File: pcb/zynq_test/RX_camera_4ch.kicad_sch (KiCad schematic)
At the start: 39 parts, among them J1601 SFW15R-2STE1LF, U1601 TCA9406DC, U1602 SN75DPHY440

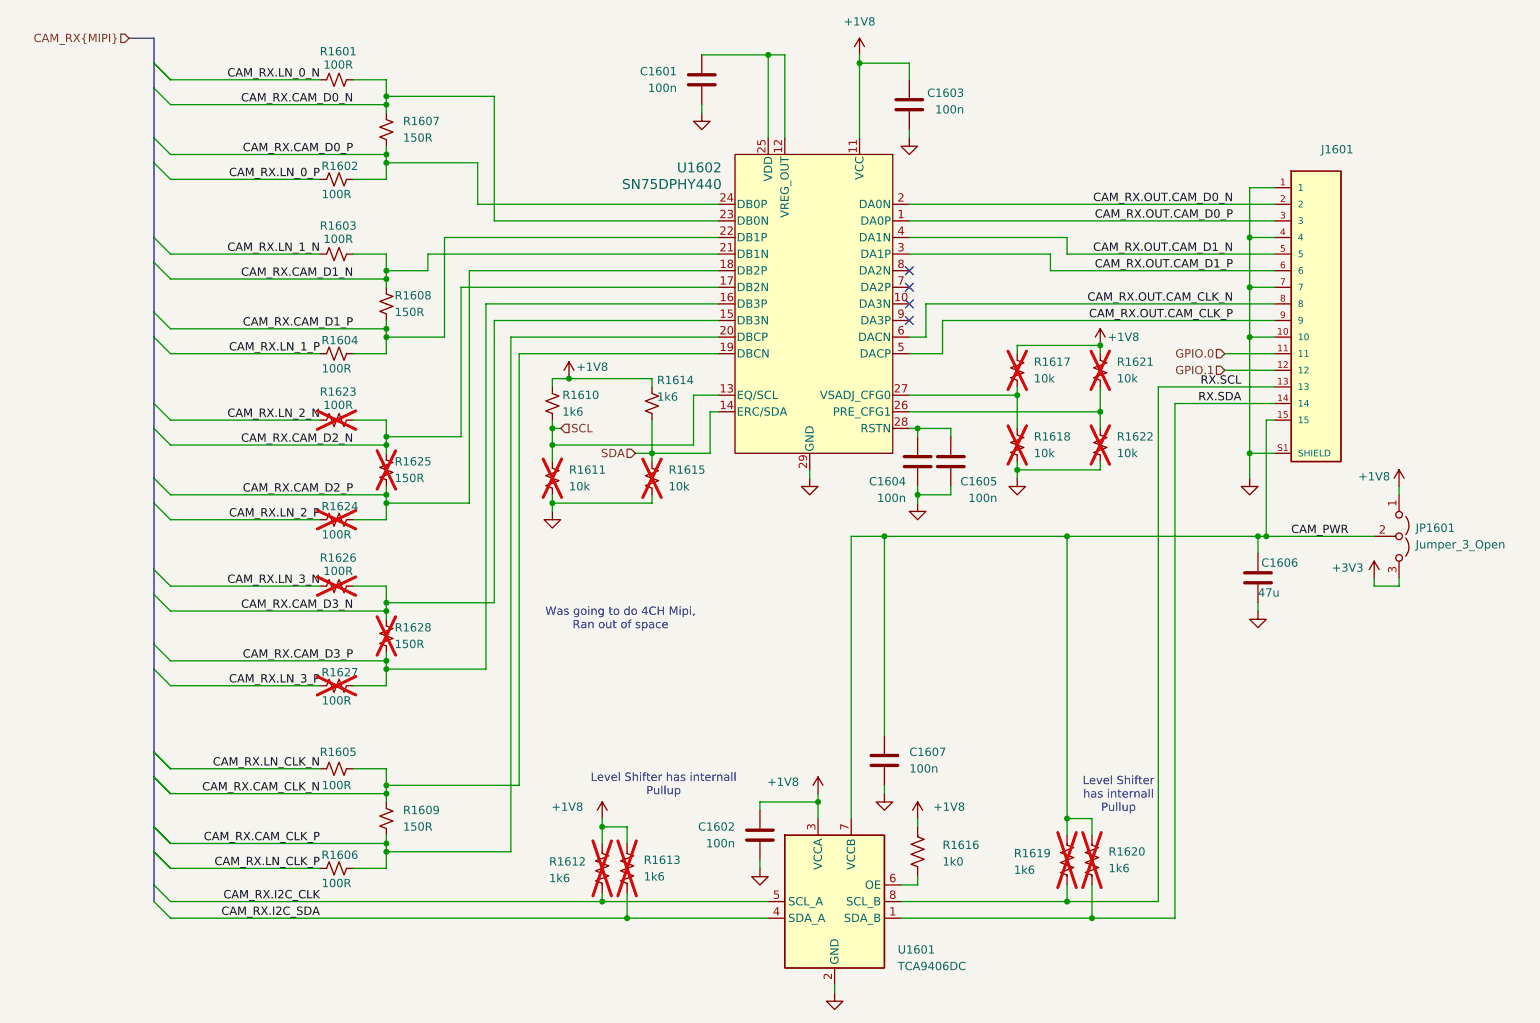
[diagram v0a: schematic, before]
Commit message: Version sent to JLCPCB
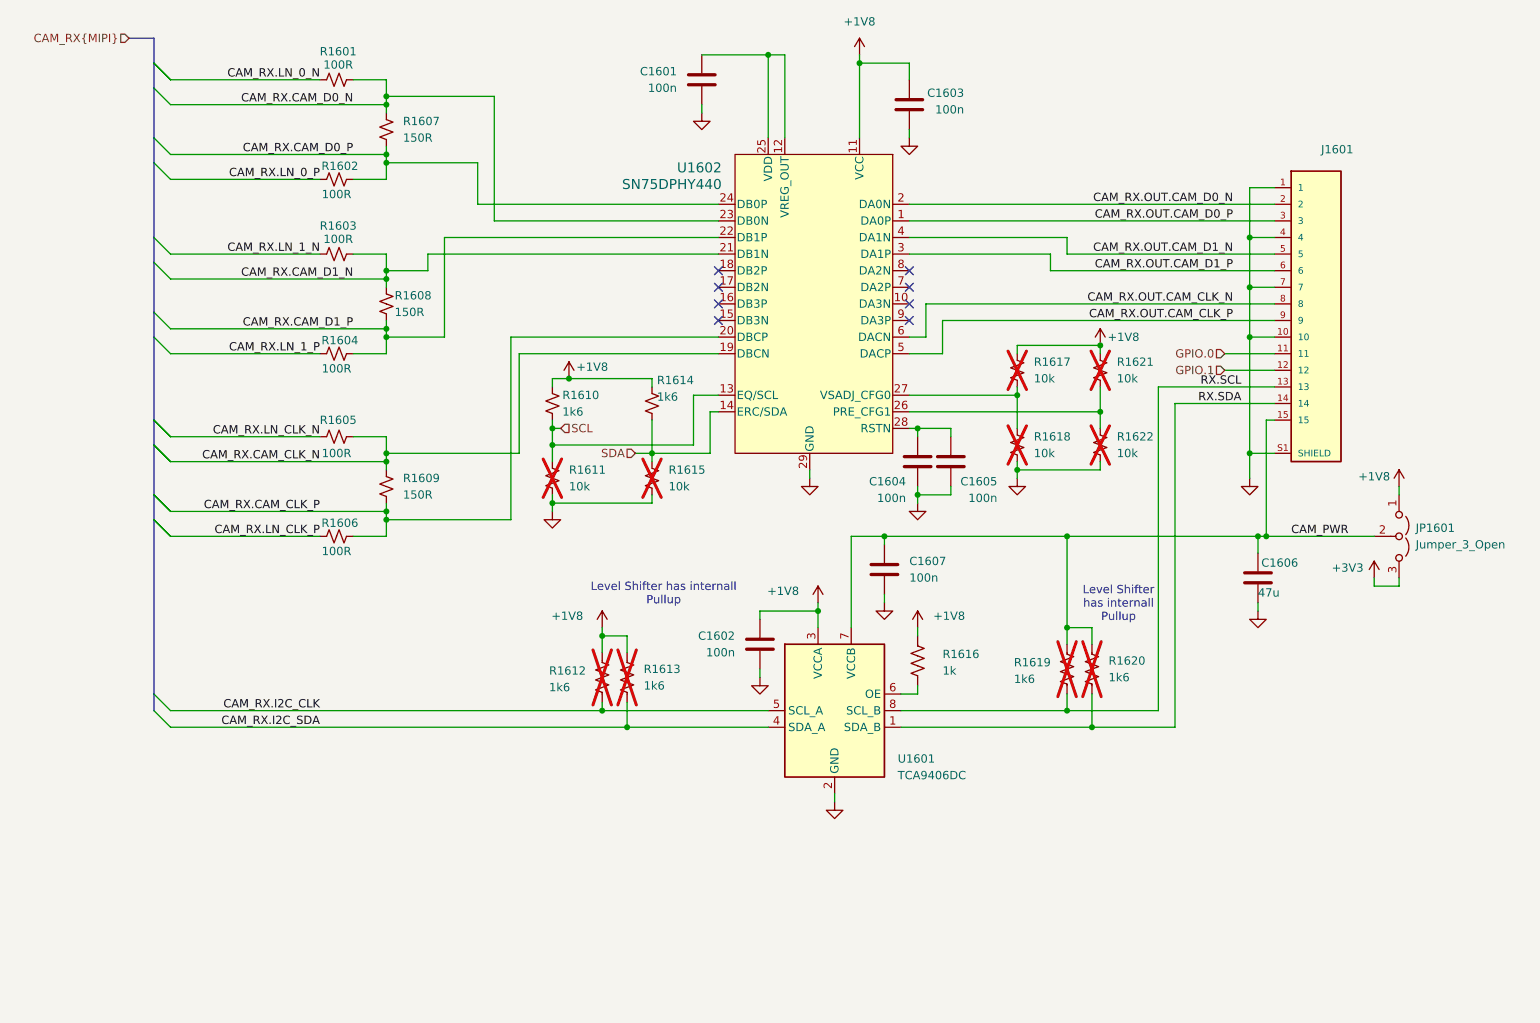
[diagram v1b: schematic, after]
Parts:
- removed R1623, R1624, R1626, R1627: 100R, Resistor_SMD:R_0402_1005Metric, symbol Device:R_Small_US
- removed R1625, R1628: 150R, Resistor_SMD:R_0402_1005Metric, symbol Device:R_Small_US
- C1601, C1602, C1603, C1604, C1605, C1607: JLCPCB Part# (none) -> C1525; PART_NUMBER (none) -> CL05B104KO5NNNC
- C1606: JLCPCB Part# (none) -> C525654; PART_NUMBER (none) -> CL32A476KPJNNNE
- J1601: JLCPCB Part# (none) -> C3167933; PART_NUMBER (none) -> SFW15R-2STE1LF
- R1601, R1602, R1603, R1604, R1605, R1606: JLCPCB Part# (none) -> C159871; PART_NUMBER (none) -> RK73B1ETTP101J
- R1607, R1608, R1609: JLCPCB Part# (none) -> C412976; PART_NUMBER (none) -> ERJ2GEJ151X
- R1610, R1614: JLCPCB Part# (none) -> C412995; PART_NUMBER (none) -> ERJ2GEJ162X
- R1611, R1615, R1617, R1618, R1621, R1622: PART_NUMBER (none) -> ERJ2RKF1002X
- R1612, R1613, R1619, R1620: PART_NUMBER (none) -> ERJ2GEJ162X
- R1616: value 1k0 -> 1k; JLCPCB Part# (none) -> C242161; PART_NUMBER (none) -> ERJ2RKF1001X
- U1601: JLCPCB Part# (none) -> C840107; PART_NUMBER (none) -> TCA9406DCUR
- U1602: JLCPCB Part# (none) -> C2863793; PART_NUMBER (none) -> SN75DPHY440SSRHRR
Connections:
- net CAM_RX.CAM_D2_N: no longer names the net of U1602.17 (DB2N)
- net CAM_RX.CAM_D2_P: no longer names the net of U1602.18 (DB2P)
- net CAM_RX.CAM_D3_N: no longer names the net of U1602.15 (DB3N)
- net CAM_RX.CAM_D3_P: no longer names the net of U1602.16 (DB3P)
- no-connect marks 4 -> 8
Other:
- note removed: "Was going to do 4CH Mipi, Ran out of space"
- moved on the sheet: C1602, C1607, R1605, R1606, R1609, R1612, R1613, R1616, R1619, R1620, U1601
